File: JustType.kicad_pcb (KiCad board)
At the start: 2 copper layers, 151.2 x 107.3 mm, 46 parts, among them SW1 SW_Push, SW10 SW_Push, SW11 SW_Push, SW12 SW_Push, SW13 SW_Push, SW14 SW_Push, SW15 SW_Push, SW16 SW_Push, SW17 SW_Push, SW18 SW_Push, SW19 SW_Push, SW2 SW_Push, SW20 SW_Push, SW21 SW_Push, SW22 SW_Push, SW3 SW_Push, SW4 SW_Push, SW5 SW_Push, SW6 SW_Push, SW7 SW_Push, SW8 SW_Push, SW9 SW_Push, U1 ProMicro

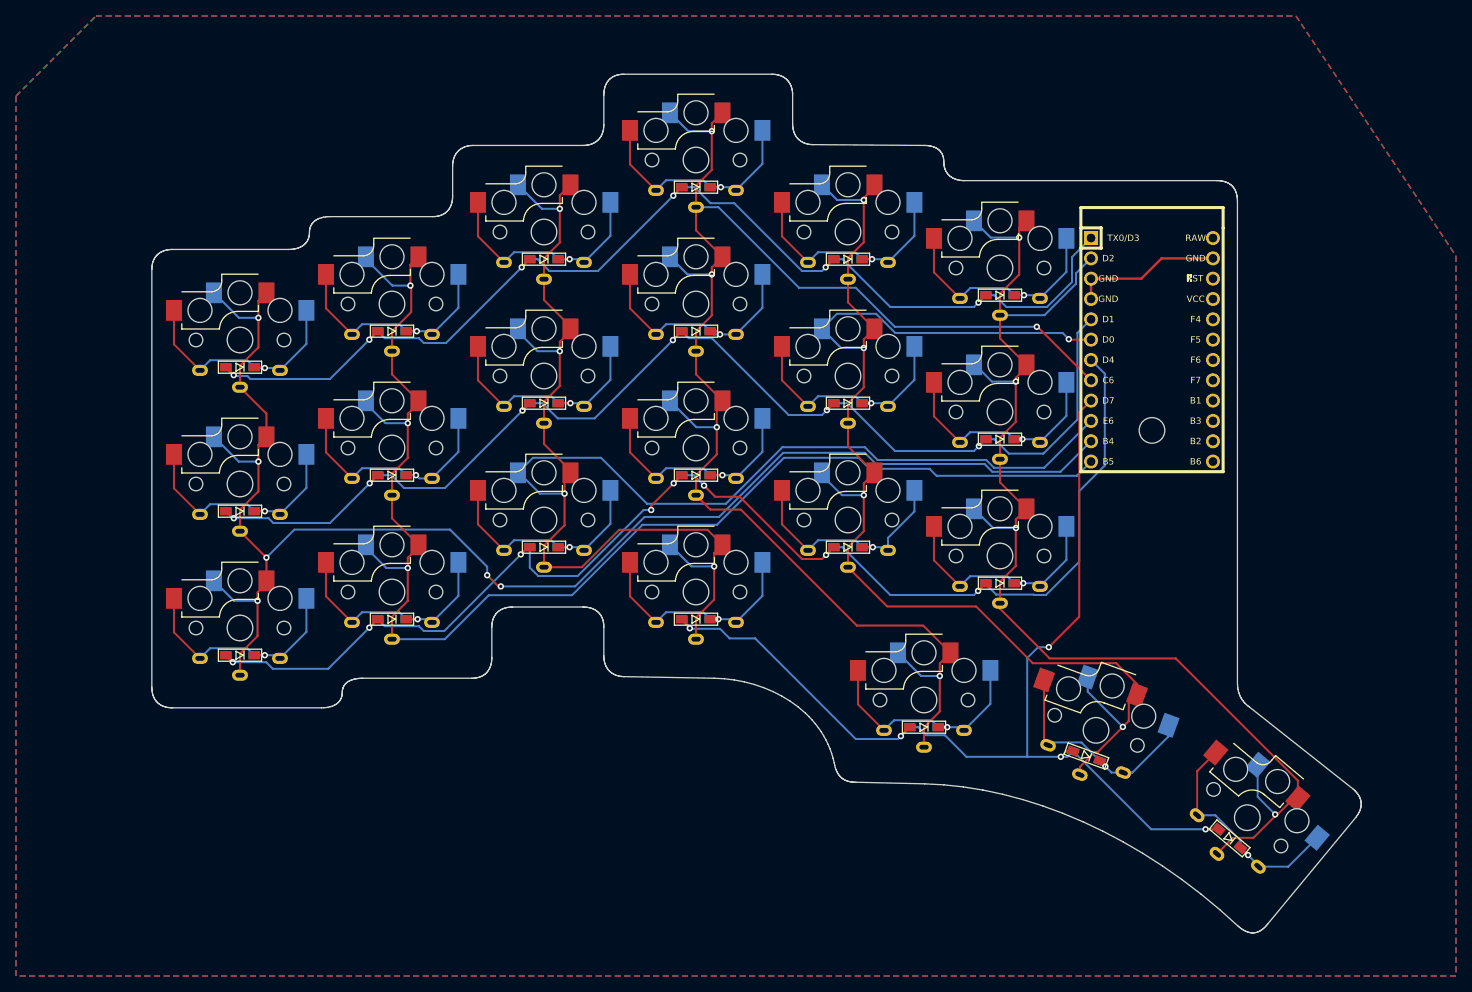
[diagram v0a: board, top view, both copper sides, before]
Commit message: validating
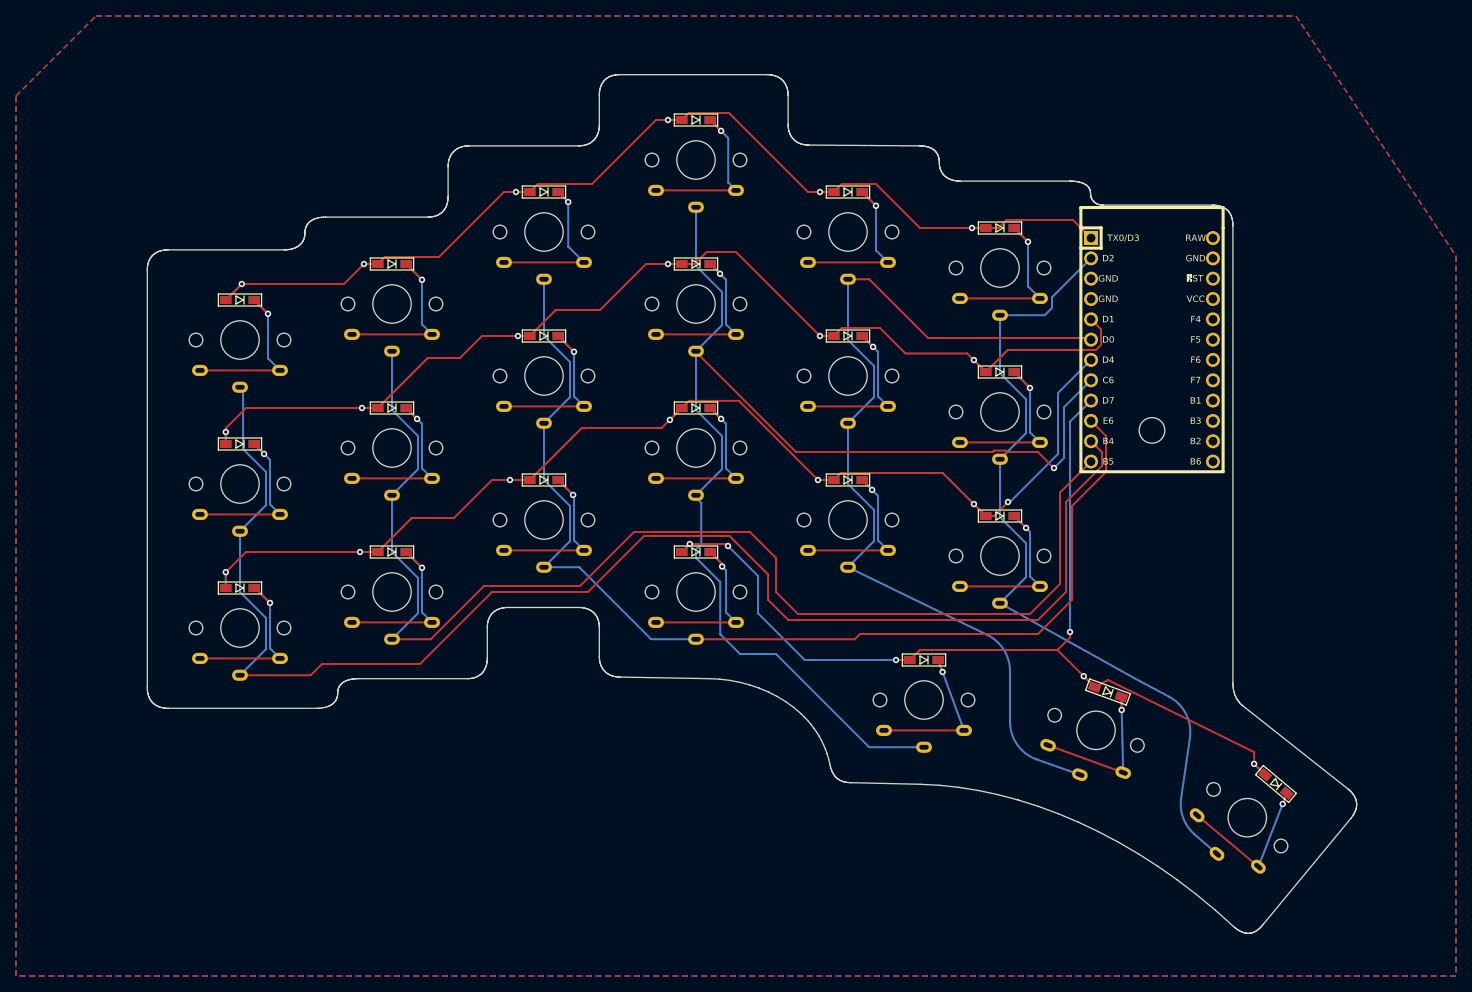
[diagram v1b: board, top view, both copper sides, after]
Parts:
- SW1, SW10, SW11, SW12, SW13, SW14, SW15, SW16, SW17, SW18, SW19, SW2, SW20, SW21, SW22, SW3, SW4, SW5, SW6, SW7, SW8, SW9: footprint keyboard_jsa:ChocV1_Solder_Reverse -> keyboard_jsa:ChocV2_Solder_2side_v1; moved to F.Cu
- moved D22 8.94 mm to (181.5, 128.5)
- moved D21 8.44 mm to (160.5, 117.0)
- moved D1 8.40 mm to (52.0, 68.0)
- moved D10 8.40 mm to (109.0, 63.5)
- moved D11 8.40 mm to (128.0, 72.5)
- moved D12 8.40 mm to (147.0, 77.0)
- moved D13 8.40 mm to (52.0, 104.0)
- moved D14 8.40 mm to (71.0, 99.5)
- moved D15 8.40 mm to (90.0, 90.5)
- moved D16 8.40 mm to (109.0, 81.5)
- moved D17 8.40 mm to (128.0, 90.5)
- moved D18 8.40 mm to (147.0, 95.0)
- moved D19 8.40 mm to (109.0, 99.5)
- moved D2 8.40 mm to (71.0, 63.5)
- moved D20 8.40 mm to (137.5, 113.0)
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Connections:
- U1 pad 21: VCC -> unconnected-(U1-VCC-Pad21)
- U1 pad 23: GND -> unconnected-(U1-GND-Pad23)
- U1 pad 3: GND -> unconnected-(U1-GND-Pad3)
- U1 pad 4: GND -> unconnected-(U1-GND-Pad4)
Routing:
- net Col 4: track 201.4 -> 138.1 mm, vias 4 -> 0
- net Col 2: track 173.9 -> 117.6 mm, vias 5 -> 0
- net Col 1: track 157.9 -> 103.0 mm, vias 4 -> 0
- net Col 3: track 192.1 -> 155.7 mm, vias 5 -> 1
- net GND: track 18.8 -> 0.00 mm
- net Row 3: track 169.5 -> 151.1 mm, vias 8 -> 7
- net Col 5: track 173.6 -> 155.6 mm, vias 3 -> 0
- net Col 6: track 192.4 -> 180.8 mm, vias 6 -> 0
- net Net-(D20-K): track 29.9 -> 21.0 mm
- net Net-(D22-K): track 29.9 -> 21.3 mm
- net Row 2: track 151.8 -> 143.2 mm
- net Net-(D21-K): track 29.4 -> 21.1 mm
- net Net-(D10-K): track 30.2 -> 21.9 mm
- net Net-(D3-K): track 30.2 -> 21.9 mm
- net Net-(D16-K): track 30.3 -> 22.1 mm
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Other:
- outline, holes or cut-outs redrawn
- board text added: "Justtype R7 2024-08"
- board text removed: "Justtype R5 2024-07"
